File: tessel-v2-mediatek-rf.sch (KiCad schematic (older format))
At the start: 43 parts, among them J501 CONN_01X01, J502 CONN_01X01, T501 2450BL15B100, T502 2450BL15B100, U201 MT7620N

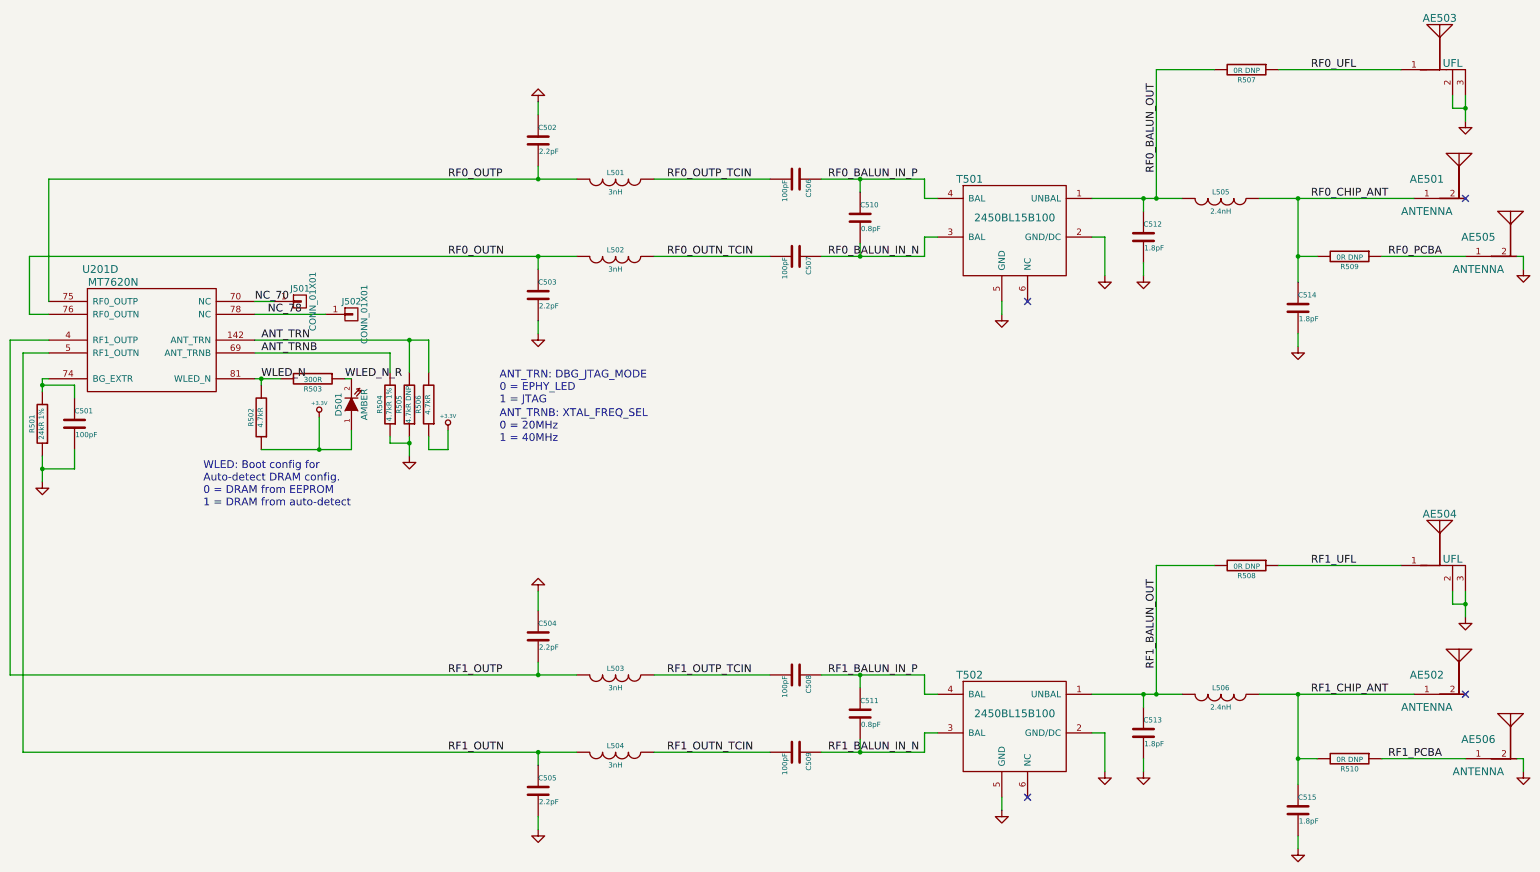
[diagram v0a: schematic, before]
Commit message: cross check with jia
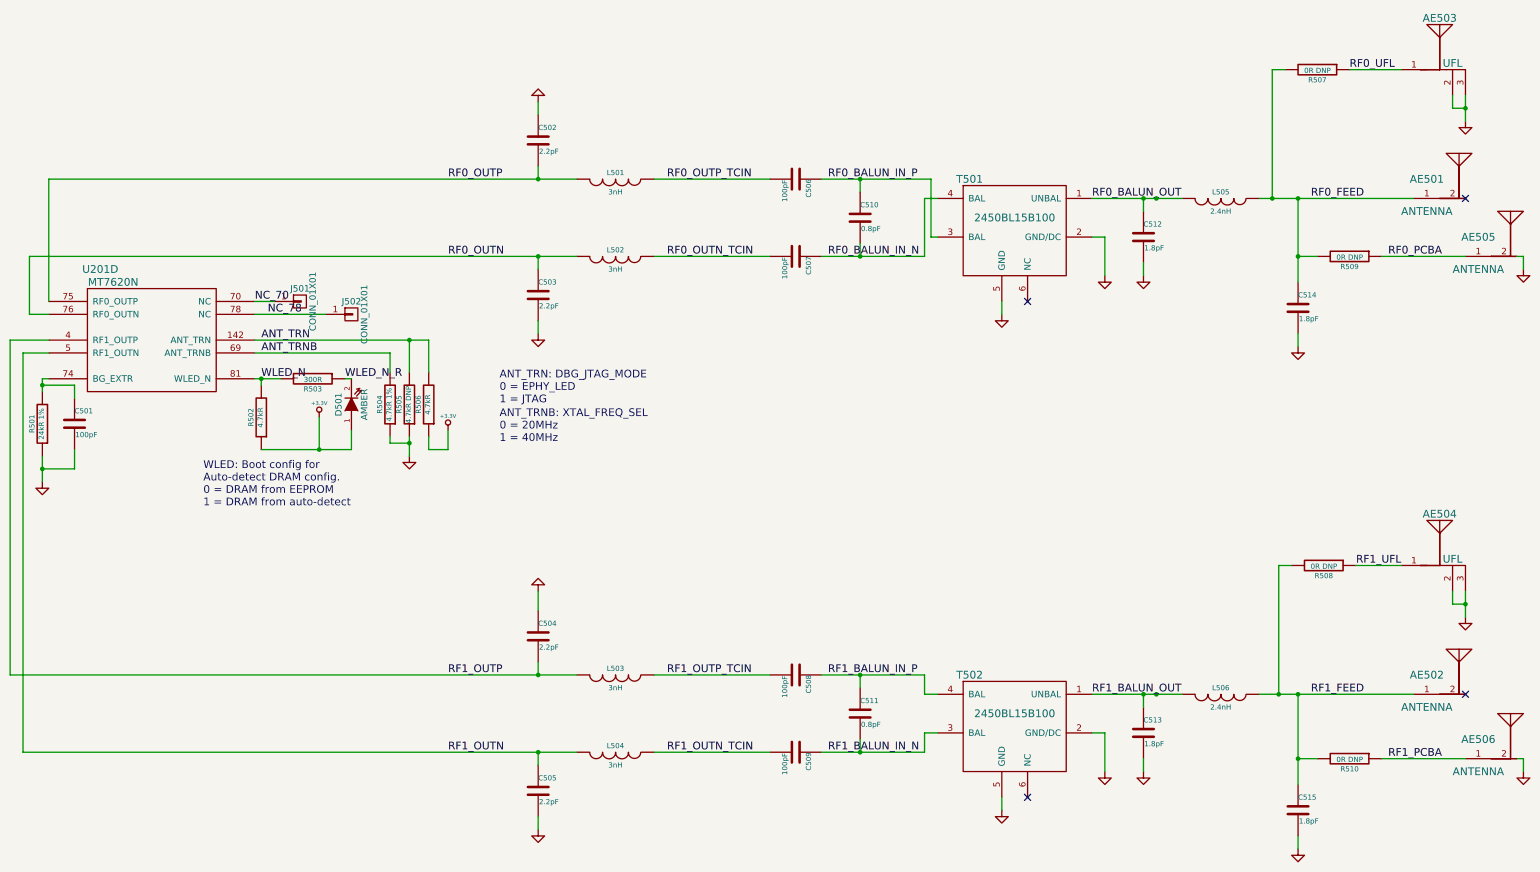
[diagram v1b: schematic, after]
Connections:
- net RF0_BALUN_IN_N: now also T501.4 (BAL); no longer T501.3 (BAL)
- net RF0_BALUN_IN_P: now also T501.3 (BAL); no longer T501.4 (BAL)
- net RF0_BALUN_OUT: no longer R507.2
- net RF1_BALUN_OUT: no longer R508.2
- net RF0_CHIP_ANT renamed RF0_FEED
- net RF0_FEED: now also R507.2
- net RF1_CHIP_ANT renamed RF1_FEED
- net RF1_FEED: now also R508.2
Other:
- moved on the sheet: R507, R508
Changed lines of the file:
@@
 L R R507
 U 1 1 549247BD
-P 11400 2750
-F 0 "R507" V 11480 2750 40  0000 C CNN
-F 1 "0R DNP" V 11407 2751 40  0000 C CNN
-F 2 "tm-kicad-lib:SMD-0402" V 11330 2750 30  0001 C CNN
-F 3 "" H 11400 2750 30  0000 C CNN
-	1    11400 2750
+P 11950 2750
+F 0 "R507" V 12030 2750 40  0000 C CNN
+F 1 "0R DNP" V 11957 2751 40  0000 C CNN
+F 2 "tm-kicad-lib:SMD-0402" V 11880 2750 30  0001 C CNN
+F 3 "" H 11950 2750 30  0000 C CNN
+	1    11950 2750
 	0    1    1    0
 $EndComp
@@
 Text Label 5200 4200 0    60   ~ 0
 RF0_OUTN
-Text Label 11900 2750 0    60   ~ 0
+Text Label 12200 2750 0    60   ~ 0
 RF0_UFL
-Text Label 10700 3550 1    60   ~ 0
+Text Label 10200 3750 0    60   ~ 0
 RF0_BALUN_OUT
 Text Label 11900 3750 0    60   ~ 0
-RF0_CHIP_ANT
+RF0_FEED
 Text Label 6900 3600 0    60   ~ 0
 RF0_OUTP_TCIN
@@
 L R R508
 U 1 1 5492F3FF
-P 11400 6600
-F 0 "R508" V 11480 6600 40  0000 C CNN
-F 1 "0R DNP" V 11407 6601 40  0000 C CNN
-F 2 "tm-kicad-lib:SMD-0402" V 11330 6600 30  0001 C CNN
-F 3 "" H 11400 6600 30  0000 C CNN
-	1    11400 6600
+P 12000 6600
+F 0 "R508" V 12080 6600 40  0000 C CNN
+F 1 "0R DNP" V 12007 6601 40  0000 C CNN
+F 2 "tm-kicad-lib:SMD-0402" V 11930 6600 30  0001 C CNN
+F 3 "" H 12000 6600 30  0000 C CNN
+	1    12000 6600
 	0    1    1    0
 $EndComp
@@
 Text Label 5200 8050 0    60   ~ 0
 RF1_OUTN
-Text Label 11900 6600 0    60   ~ 0
+Text Label 12250 6600 0    60   ~ 0
 RF1_UFL
-Text Label 10700 7400 1    60   ~ 0
+Text Label 10200 7600 0    60   ~ 0
 RF1_BALUN_OUT
 Text Label 11900 7600 0    60   ~ 0
-RF1_CHIP_ANT
+RF1_FEED
 Text Label 6900 7450 0    60   ~ 0
 RF1_OUTP_TCIN
@@
 Connection ~ 5900 3600
 Wire Wire Line
-	11150 2750 10700 2750
+	11700 2750 11600 2750
 Connection ~ 10700 3750
 Wire Wire Line
 	11500 3750 12700 3750
 Wire Wire Line
-	11650 2750 12600 2750
+	12200 2750 12600 2750
 Wire Wire Line
 	11800 7600 11800 8300
@@
 	5900 7350 5900 7450
 Connection ~ 5900 7450
-Wire Wire Line
-	11150 6600 10700 6600
 Connection ~ 10700 7600
 Wire Wire Line
 	11500 7600 12700 7600
 Wire Wire Line
-	11650 6600 12600 6600
+	12250 6600 12600 6600
 Wire Wire Line
 	2100 4550 2100 3600
@@
 	10200 3750 10900 3750
 Wire Wire Line
-	8100 3600 8900 3600
-Wire Wire Line
-	8900 3600 8900 3750
-Wire Wire Line
-	8100 4200 8900 4200
-Wire Wire Line
-	8900 4200 8900 4050
-Wire Wire Line
-	8900 3750 9000 3750
-Wire Wire Line
-	8900 4050 9000 4050
+	8100 3600 8950 3600
+Wire Wire Line
+	8900 4200 8100 4200
+Wire Wire Line
+	8900 3750 8900 4200
 $Comp
 L 2450BL15B100 T502
@@
 Text Label 8150 3600 0    60   ~ 0
 RF0_BALUN_IN_P
-Wire Wire Line
-	10700 2750 10700 3750
-Wire Wire Line
-	10700 6600 10700 7600
 Connection ~ 11800 8100
 Connection ~ 11800 4200
+Wire Wire Line
+	11600 2750 11600 3750
+Connection ~ 11600 3750
+Wire Wire Line
+	11750 6600 11650 6600
+Wire Wire Line
+	11650 6600 11650 7600
+Connection ~ 11650 7600
+Wire Wire Line
+	8900 3750 9000 3750
+Wire Wire Line
+	9000 4050 8950 4050
+Wire Wire Line
+	8950 4050 8950 3600
 $EndSCHEMATC
